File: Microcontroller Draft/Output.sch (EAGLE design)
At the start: 33 parts, among them Q1 IRF9530, Q2 IRF9530, Q3 IRF9530, T1 BC547, T2 BC547, T3 BC547, U1 TLV2372IP

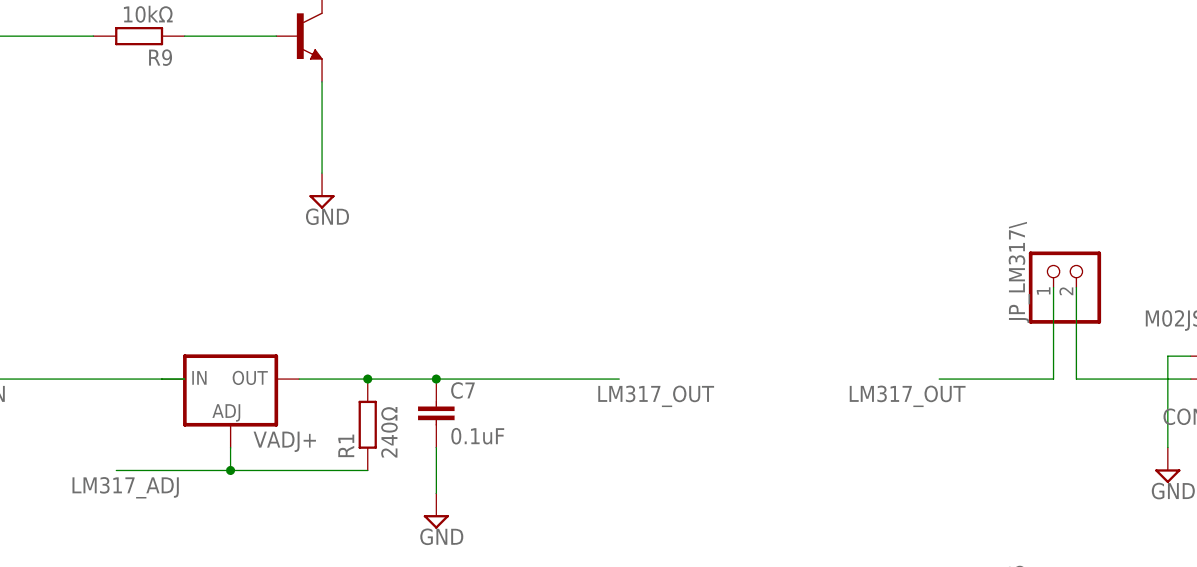
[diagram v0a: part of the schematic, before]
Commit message: Fixed some errors
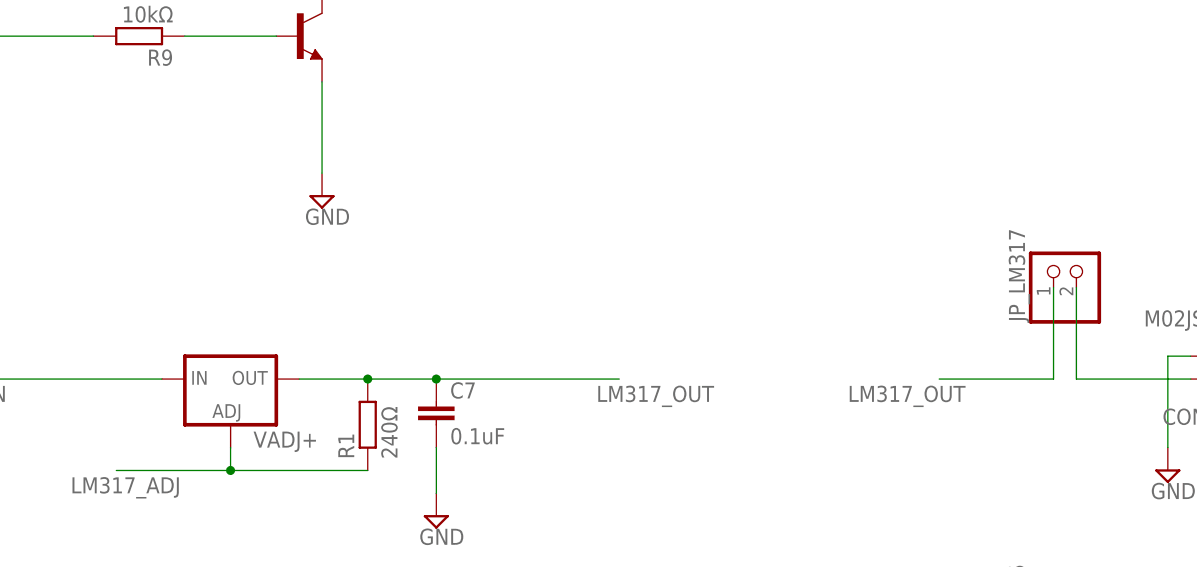
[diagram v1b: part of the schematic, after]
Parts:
- renumbered JP_LM317\ to JP_LM317
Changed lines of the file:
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@@
 <part name="SUPPLY9" library="supply2" deviceset="GND" device=""/>
 <part name="C5" library="rcl" deviceset="C-EU" device="025-025X050" value="0.1uF"/>
-<part name="JP_LM317\" library="pinhead" deviceset="PINHD-1X2" device=""/>
+<part name="JP_LM317" library="pinhead" deviceset="PINHD-1X2" device=""/>
 <part name="JP_7805" library="pinhead" deviceset="PINHD-1X2" device=""/>
 <part name="JP_LD33V" library="pinhead" deviceset="PINHD-1X2" device=""/>
@@
 <instance part="SUPPLY9" gate="GND" x="45.72" y="88.9"/>
 <instance part="C5" gate="G$1" x="45.72" y="99.06"/>
-<instance part="JP_LM317\" gate="G$1" x="307.34" y="111.76" rot="R90"/>
+<instance part="JP_LM317" gate="G$1" x="307.34" y="111.76" rot="R90"/>
 <instance part="JP_7805" gate="G$1" x="307.34" y="76.2" rot="R90"/>
 <instance part="JP_LD33V" gate="G$1" x="307.34" y="40.64" rot="R90"/>
@@
 </segment>
 <segment>
-<pinref part="JP_LM317\" gate="G$1" pin="1"/>
+<pinref part="JP_LM317" gate="G$1" pin="1"/>
 <wire x1="304.8" y1="109.22" x2="304.8" y2="99.06" width="0.1524" layer="91"/>
 <wire x1="304.8" y1="99.06" x2="292.1" y2="99.06" width="0.1524" layer="91"/>
@@
 <net name="LM317_IN" class="0">
 <segment>
-<wire x1="205.74" y1="99.06" x2="208.28" y2="99.06" width="0.1524" layer="91"/>
 <pinref part="VADJ+" gate="A" pin="IN"/>
 <wire x1="205.74" y1="99.06" x2="180.34" y2="99.06" width="0.1524" layer="91"/>
@@
 <net name="N$7" class="0">
 <segment>
-<pinref part="JP_LM317\" gate="G$1" pin="2"/>
+<pinref part="JP_LM317" gate="G$1" pin="2"/>
 <wire x1="307.34" y1="109.22" x2="307.34" y2="99.06" width="0.1524" layer="91"/>
 <wire x1="307.34" y1="99.06" x2="320.04" y2="99.06" width="0.1524" layer="91"/>
